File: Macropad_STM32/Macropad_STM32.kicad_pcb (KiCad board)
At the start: 4 copper layers, 183.3 x 93.4 mm, 209 parts, among them J1 USB_C_Receptacle_USB2.0, J10 Encoders + LED, J12 Power Connector, J13 Conn_01x04_Socket, J14 Conn_01x04_Socket, J16 Conn_01x04_Socket, J17 Conn_01x04_Socket, J18 Conn_01x04_Socket, J19 Conn_01x04_Socket, J2 USB_A, J21 Matrix, J22 Encoders + LED, J3 JTAG, J4 Conn_01x04_Socket, J5 Conn_01x04_Socket, J6 USB_C_Receptacle_USB2.0, J7 Power Connector, J8 USB_A, J9 Matrix, K1 Kailh Hotswap Socket, K10 Kailh Hotswap Socket, K11 Kailh Hotswap Socket, K12 Kailh Hotswap Socket, K13 Kailh Hotswap Socket, K14 Kailh Hotswap Socket, K15 Kailh Hotswap Socket, K16 Kailh Hotswap Socket, K2 Kailh Hotswap Socket, K3 Kailh Hotswap Socket, K4 Kailh Hotswap Socket, K5 Kailh Hotswap Socket, K6 Kailh Hotswap Socket, K7 Kailh Hotswap Socket, K8 Kailh Hotswap Socket, K9 Kailh Hotswap Socket, SW1 SW_Push, SW2 EC11 Encoder, SW3 EC11 Encoder, U1 STM32F103C8T6, U2 CY7C65632-28LTXCT, U3 AMS1117-3.3, U4 USBLC6-2SC6, U6 USBLC6-2SC6, U7 USBLC6-2SC6, U8 USBLC6-2SC6, Y1 16MHz, Y2 12MHz

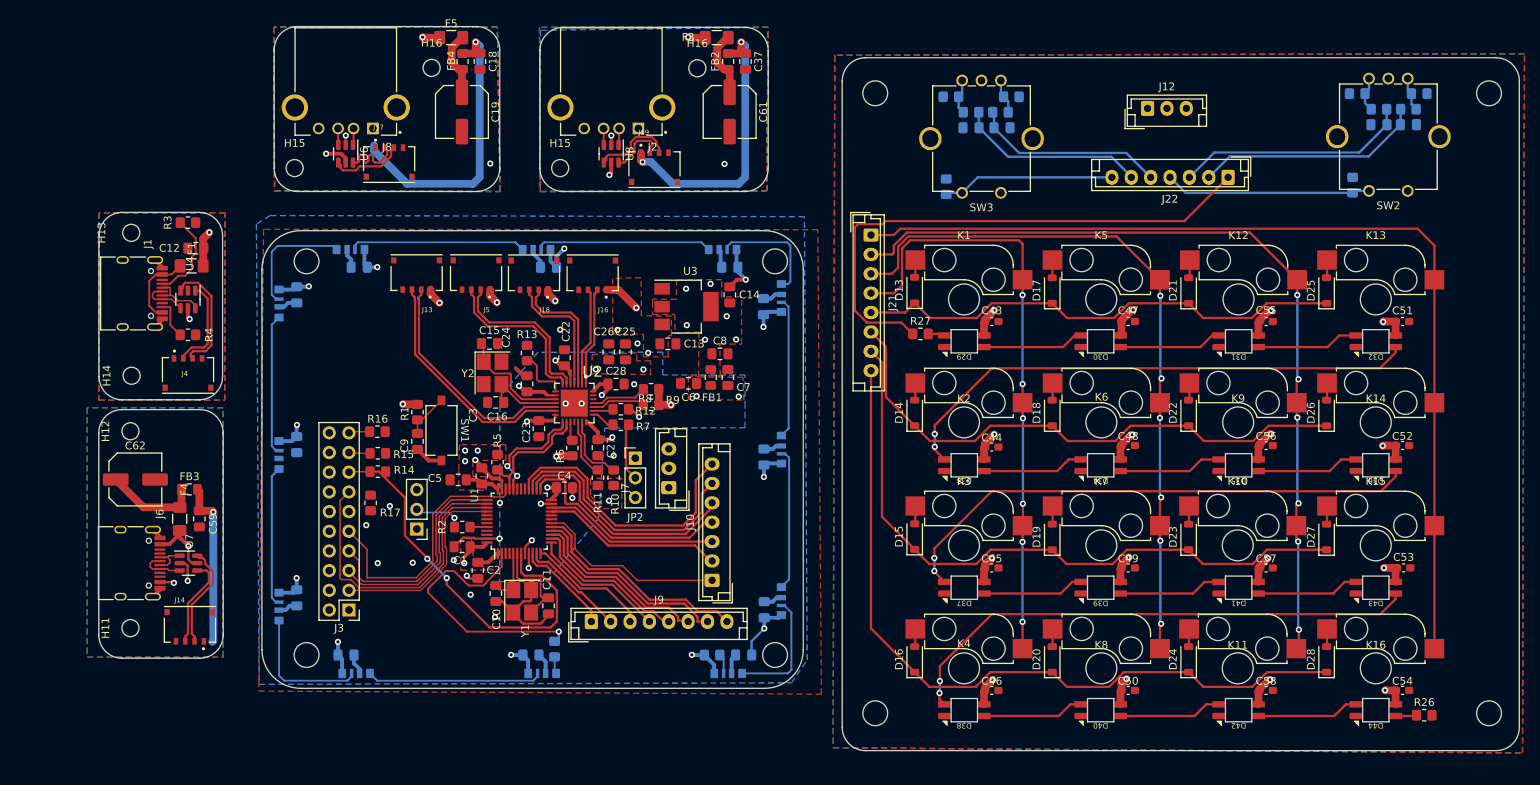
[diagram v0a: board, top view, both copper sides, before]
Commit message: Nearly finished Todo: - Fix silkscreen - Final check
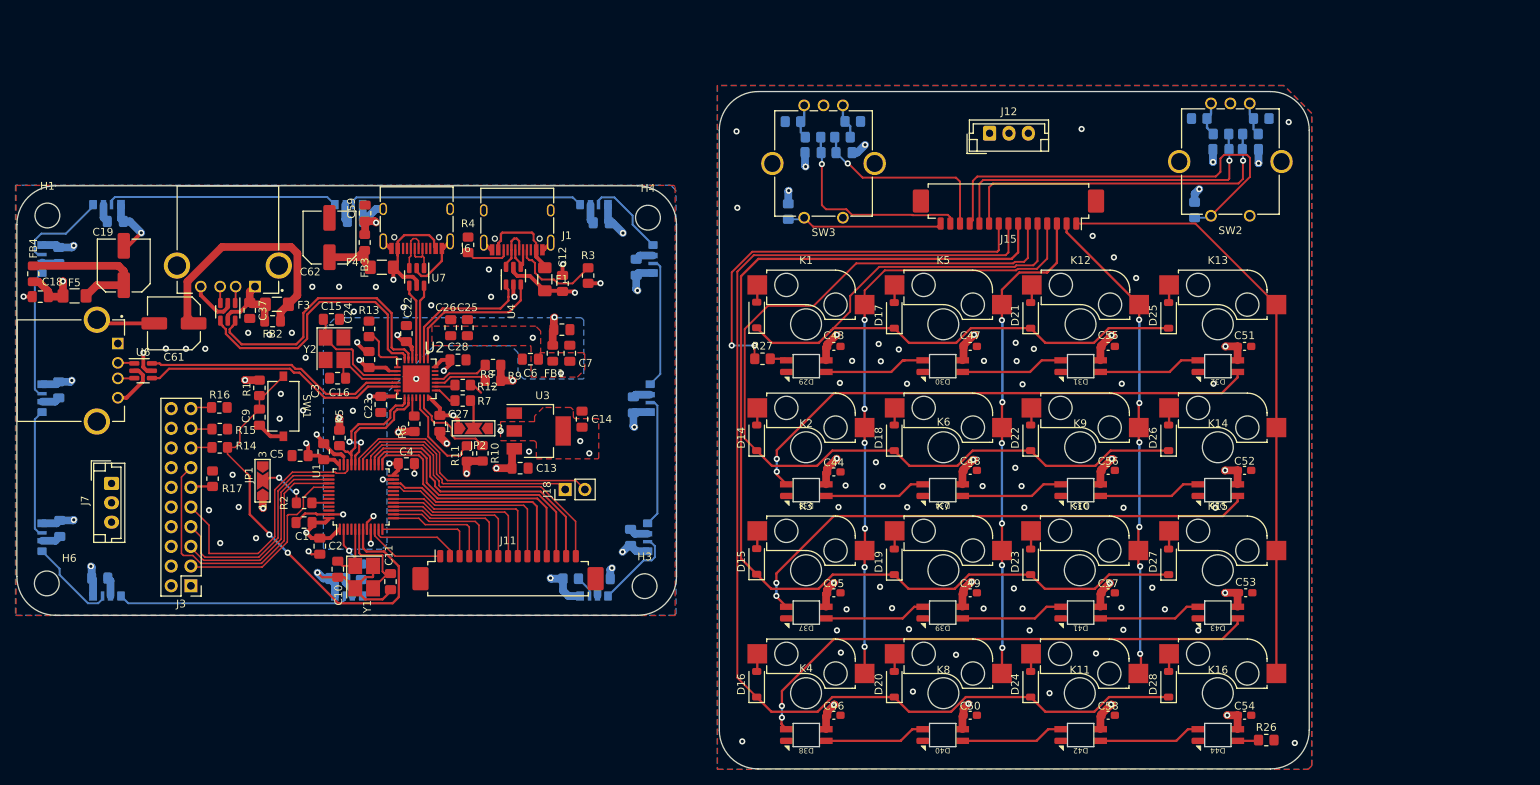
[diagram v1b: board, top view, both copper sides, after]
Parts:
- removed H11, H12, H13, H14, H15 (x2), H16 (x2): MountingHole, MountingHole:MountingHole_2.2mm_M2
- removed H2, H5, H7, H8: MountingHole, MountingHole:MountingHole_3.2mm_M3_DIN965
- removed J10, J22: Encoders + LED, Connector_JST:JST_EH_B7B-EH-A_1x07_P2.50mm_Vertical
- removed J13, J14, J16, J17, J19, J4, J5: Conn_01x04_Socket, SK6812SIDE:MOLEX_0781710004
- removed J21, J9: Matrix, Connector_JST:JST_EH_B8B-EH-A_1x08_P2.50mm_Vertical
- added J11: 533981571, Connector_Molex:Molex_PicoBlade_53261-1571_1x15-1MP_P1.25mm_Horizontal, F.Cu at (127.0, 118.7)
- added J15: 533981571, Connector_Molex:Molex_PicoBlade_53261-1571_1x15-1MP_P1.25mm_Horizontal, F.Cu at (191.6, 71.0)
- J18: value Conn_01x04_Socket -> Conn_01x02_Socket; footprint SK6812SIDE:MOLEX_0781710004 -> Connector_PinHeader_2.54mm:PinHeader_1x02_P2.54mm_Vertical
- JP1, JP2: footprint Connector_PinHeader_2.54mm:PinHeader_1x03_P2.54mm_Vertical -> Jumper:SolderJumper-3_P2.0mm_Open_TrianglePad1.0x1.5mm_NumberLabels
- moved H6 196.6 mm to (67.5, 119.8)
- moved H1 109.7 mm to (67.6, 72.3)
- moved C61 76.7 mm to (83.9, 86.3), turned to 180 degrees
- moved J7 71.9 mm to (75.8, 106.9), turned to -90 degrees
- moved C37 71.6 mm to (93.7, 84.6)
- moved FB2 67.7 mm to (96.6, 86.0), turned to 180 degrees
- moved F3 66.4 mm to (97.2, 83.8)
- moved C18 64.3 mm to (66.6, 82.8), turned to 180 degrees
- moved FB4 61.8 mm to (65.7, 79.9), turned to -90 degrees
- moved H3 60.5 mm to (144.6, 120.2)
- moved F5 58.9 mm to (71.1, 82.7)
- moved J6 58.1 mm to (115.2, 72.5), turned to 180 degrees
- moved J2 53.5 mm to (90.9, 81.5)
- moved U8 53.5 mm to (90.8, 84.8)
- moved R3 52.1 mm to (137.3, 80.1), turned to -90 degrees
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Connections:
- C12 pad 1: /USB_UP_GND -> GND
- C12 pad 2: /VBUS_IN -> VBUS
- C18 pad 1: Net-(J17-Pin_1) -> VBUS
- C18 pad 2: /USBHUB/D2_GND -> GND
- C19 pad 2: /USBHUB/D2_GND -> GND
- C37 pad 1: Net-(J19-Pin_1) -> VBUS
- C37 pad 2: /USBHUB/D1_GND -> GND
- C39 pad 1: /Matrix/ENC_1_A -> /Matrix/ENC_1_B
- C40 pad 1: /Matrix/ENC_2_A -> /Matrix/ENC_2_B
- C43 pad 2: Net-(C43-Pad2) -> GND1
- C46 pad 2: Net-(C43-Pad2) -> GND1
- C49 pad 2: Net-(C43-Pad2) -> GND1
- C52 pad 2: Net-(C43-Pad2) -> GND1
- C59 pad 1: Net-(J14-Pin_1) -> VBUS
- C59 pad 2: /USBHUB/D3_GND -> GND
- C61 pad 2: /USBHUB/D1_GND -> GND
- C62 pad 2: /USBHUB/D3_GND -> GND
- F1 pad 2: /VBUS_IN -> VBUS
- F3 pad 1: /USBHUB/D1_VBUS -> VBUS
- F4 pad 1: /USBHUB/D3_VBUS -> VBUS
- F5 pad 1: /USBHUB/D2_VBUS -> VBUS
- FB2 pad 2: Net-(J19-Pin_1) -> VBUS
- FB3 pad 2: Net-(J14-Pin_1) -> VBUS
- FB4 pad 2: Net-(J17-Pin_1) -> VBUS
- J1 pad A1: /USB_UP_GND -> GND
- J1 pad A12: /USB_UP_GND -> GND
- J1 pad B1: /USB_UP_GND -> GND
- J1 pad B12: /USB_UP_GND -> GND
- J1 pad S1: /USB_UP_GND -> GND
- J18 pad 1: VBUS -> Net-(J18-Pin_1)
- J18 pad 2: /USBHUB/D1_D- -> Net-(J18-Pin_2)
- J2 pad 1: /USBHUB/D1_VBUS -> VBUS
- J2 pad 4: /USBHUB/D1_GND -> GND
- J2 pad 5: /USBHUB/D1_GND -> GND
- J6 pad A1: /USBHUB/D3_GND -> GND
- J6 pad A12: /USBHUB/D3_GND -> GND
- J6 pad A4: /USBHUB/D3_VBUS -> VBUS
- J6 pad A9: /USBHUB/D3_VBUS -> VBUS
- J6 pad B1: /USBHUB/D3_GND -> GND
- J6 pad B12: /USBHUB/D3_GND -> GND
- J6 pad B4: /USBHUB/D3_VBUS -> VBUS
- J6 pad B9: /USBHUB/D3_VBUS -> VBUS
- J6 pad S1: /USBHUB/D3_GND -> GND
- J8 pad 1: /USBHUB/D2_VBUS -> VBUS
- J8 pad 4: /USBHUB/D2_GND -> GND
- J8 pad 5: /USBHUB/D2_GND -> GND
- R27 pad 1: +5V -> /Matrix/Key_LED
- R3 pad 2: /USB_UP_GND -> GND
- R31 pad 2: /Matrix/ENC_1_A -> /Matrix/ENC_1_B
- R35 pad 2: /Matrix/ENC_2_A -> /Matrix/ENC_2_B
- R4 pad 2: /USB_UP_GND -> GND
- U1 pad 30: unconnected-(U1-PA9-Pad30) -> Net-(J18-Pin_1)
- U1 pad 31: unconnected-(U1-PA10-Pad31) -> Net-(J18-Pin_2)
- U4 pad 1: /UP_USB_D- -> /UP_USB_D+
- U4 pad 2: /USB_UP_GND -> GND
- U4 pad 3: /UP_USB_D+ -> /UP_USB_D-
- U4 pad 4: /USB_UP_D+ -> /USB_UP_D-
- U4 pad 5: /VBUS_IN -> VBUS
- U4 pad 6: /USB_UP_D- -> /USB_UP_D+
- U6 pad 2: /USBHUB/D2_GND -> GND
- U6 pad 4: /USBHUB/Daughter_D2_D+ -> /USBHUB/D3_D+
- U6 pad 5: /USBHUB/D2_VBUS -> VBUS
- U6 pad 6: /USBHUB/Daughter_D2_D- -> /USBHUB/D3_D-
- U7 pad 2: /USBHUB/D3_GND -> GND
- U7 pad 4: /USBHUB/Daughter_D3_D+ -> /USBHUB/D1_D+
- U7 pad 5: /USBHUB/D3_VBUS -> VBUS
- U7 pad 6: /USBHUB/Daughter_D3_D- -> /USBHUB/D1_D-
- U8 pad 2: /USBHUB/D1_GND -> GND
- U8 pad 4: /USBHUB/Daughter_D1_D+ -> /USBHUB/D2_D+
- U8 pad 5: /USBHUB/D1_VBUS -> VBUS
- U8 pad 6: /USBHUB/Daughter_D1_D- -> /USBHUB/D2_D-
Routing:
- net +5V: track 129.5 -> 59.8 mm
- net /Matrix/ROW3: track 99.1 -> 153.5 mm
- net /Matrix/Key_LED: track 0.00 -> 53.2 mm, vias 0 -> 2
- net /Matrix/ROW2: track 85.6 -> 137.8 mm
- net /Matrix/COL3: track 126.0 -> 77.8 mm
- net /Matrix/ROW1: track 72.5 -> 119.1 mm
- net GND: track 96.0 -> 141.8 mm, vias 33 -> 50
- net /Matrix/COL2: track 107.5 -> 62.7 mm
- net VBUS: track 38.9 -> 83.5 mm
- net /Matrix/ENC_1_B: track 0.00 -> 43.3 mm, vias 0 -> 1
- net Net-(J17-Pin_1): track 38.0 -> 0.00 mm, vias 1 -> 0
- net Net-(J19-Pin_1): track 37.6 -> 0.00 mm, vias 2 -> 0
- net Net-(J18-Pin_2): track 0.00 -> 35.2 mm
- net Net-(J18-Pin_1): track 0.00 -> 32.0 mm
- net /Matrix/ROW0: track 64.0 -> 94.2 mm
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- added copper zone on B.Cu, net +3V3
- added copper zone on In2.Cu, net +5V
- added copper zone on In2.Cu, net GND
- removed copper zone on In2.Cu, net +3V3
- removed copper zone on B.Cu, net +5V
- removed copper zone on B.Cu, net /USBHUB/D1_GND
- removed copper zone on F.Cu, net /USBHUB/D1_GND
- removed copper zone on In1.Cu, net /USBHUB/D1_GND
- removed copper zone on B.Cu, net /USBHUB/D1_VBUS
- removed copper zone on In2.Cu, net /USBHUB/D1_VBUS
- removed copper zone on B.Cu, net /USBHUB/D2_GND
- removed copper zone on F.Cu, net /USBHUB/D2_GND
- removed copper zone on In1.Cu, net /USBHUB/D2_GND
- removed copper zone on In2.Cu, net /USBHUB/D2_VBUS
- removed copper zone on B.Cu, net /USBHUB/D3_GND
- removed copper zone on F.Cu, net /USBHUB/D3_GND
- removed copper zone on In1.Cu, net /USBHUB/D3_GND
- removed copper zone on In2.Cu, net /USBHUB/D3_VBUS
- removed copper zone on B.Cu, net /USB_UP_GND
- removed copper zone on F.Cu, net /USB_UP_GND
- removed copper zone on In1.Cu, net /USB_UP_GND
- removed copper zone on In2.Cu, net /VBUS_IN
- removed copper zone on F.Cu, net VBUS
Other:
- board size 183.3 x 93.4 mm -> 166.8 x 87.4 mm
